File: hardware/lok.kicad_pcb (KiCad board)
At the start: 2 copper layers, 80 x 20 mm, 2 parts, among them U1 XIAO-ESP32-S3-SMD, U2 STSPIN233

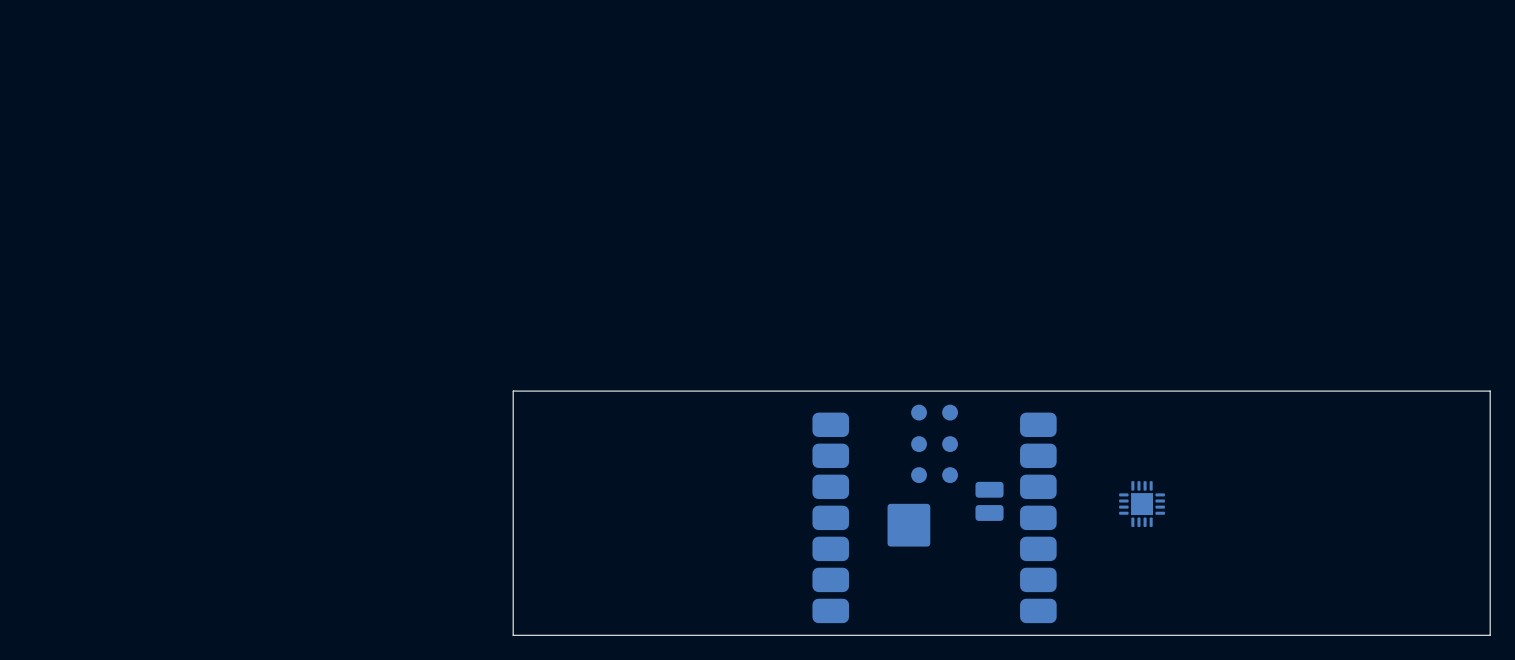
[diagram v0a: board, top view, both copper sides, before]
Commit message: update
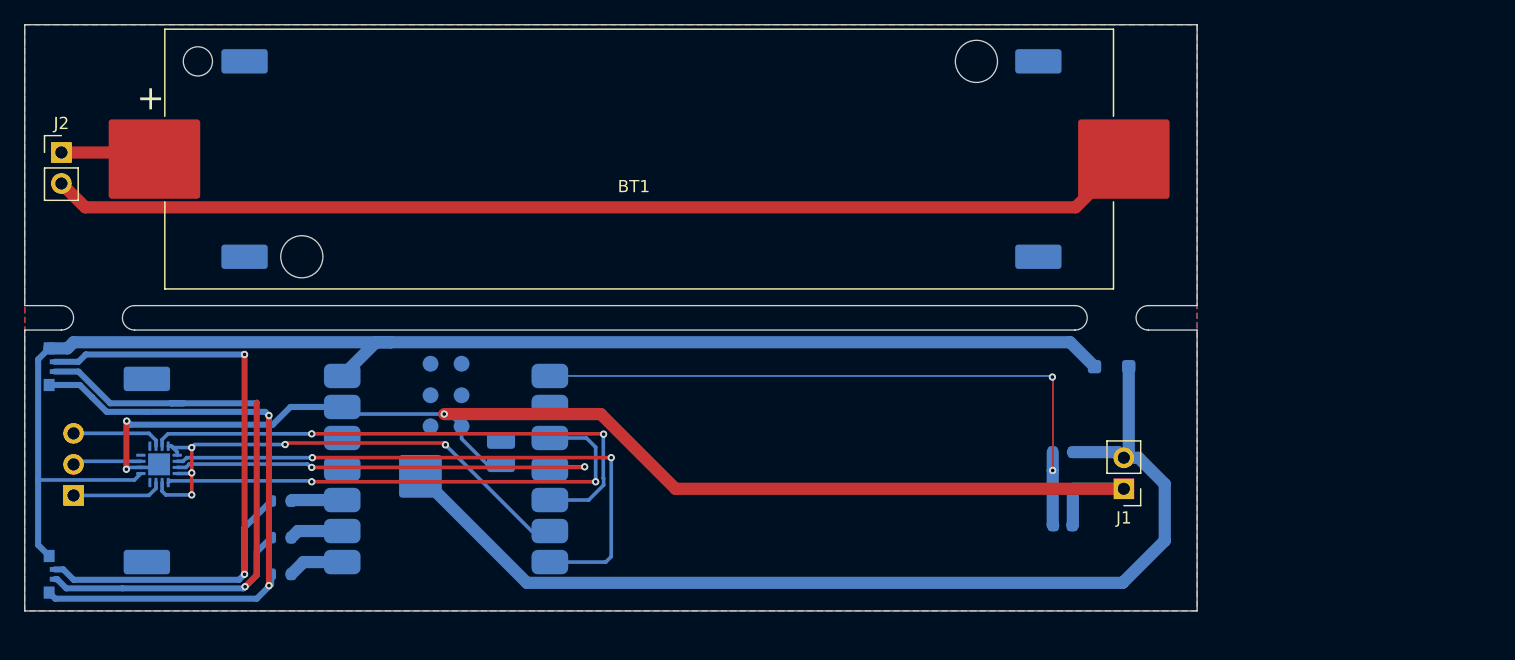
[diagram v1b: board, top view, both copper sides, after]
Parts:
- added BT1: Battery_Cell, Battery:BatteryHolder_Keystone_1042_1x18650, F.Cu at (110.3, 81.0)
- added C1: 1u, Capacitor_SMD:C_0603_1608Metric, B.Cu at (145.0, 111.0)
- added D1: D, Diode_SMD:D_SOD-123F, B.Cu at (149.0, 98.0)
- added D2: LED_ABGR, LED_SMD:LED_Kingbright_APFA3010_3x1.5mm_Horizontal, B.Cu at (62.0, 98.0)
- added D3: LED_ABGR, LED_SMD:LED_Kingbright_APFA3010_3x1.5mm_Horizontal, B.Cu at (62.0, 115.0)
- added J1: Conn_01x02_Pin, Connector_PinHeader_2.54mm:PinHeader_1x02_P2.54mm_Vertical, F.Cu at (150.0, 108.0)
- added J2: Conn_01x02_Pin, Connector_PinHeader_2.54mm:PinHeader_1x02_P2.54mm_Vertical, F.Cu at (63.0, 80.5)
- added J3: Conn_01x03_Pin, Connector_PinHeader_2.54mm:PinHeader_1x03_P2.54mm_Vertical, B.Cu at (64.0, 108.5)
- added R1: 220k, Resistor_SMD:R_0603_1608Metric, B.Cu at (145.0, 105.0)
- added R2: 47k, Resistor_SMD:R_0603_1608Metric, B.Cu at (145.0, 108.0)
- added R3: 100, Resistor_SMD:R_0603_1608Metric, B.Cu at (81.0, 109.0)
- added R4: 100, Resistor_SMD:R_0603_1608Metric, B.Cu at (81.0, 112.0)
- added R5: 100, Resistor_SMD:R_0603_1608Metric, B.Cu at (81.0, 115.0)
- added TP3: TestPoint, TestPoint:TestPoint_Keystone_5019_Miniature, B.Cu at (70.0, 114.0)
- added TP4: TestPoint, TestPoint:TestPoint_Keystone_5019_Miniature, B.Cu at (70.0, 99.0)
- added TP5: TestPoint, TestPoint:TestPoint_Keystone_5019_Miniature, B.Cu at (143.0, 73.0)
- added TP6: TestPoint, TestPoint:TestPoint_Keystone_5019_Miniature, B.Cu at (143.0, 89.0)
- added TP7: TestPoint, TestPoint:TestPoint_Keystone_5019_Miniature, B.Cu at (78.0, 89.0)
- added TP8: TestPoint, TestPoint:TestPoint_Keystone_5019_Miniature, B.Cu at (78.0, 73.0)
- moved U2 80.6 mm to (71.0, 106.0), turned to 90 degrees
- moved U1 40.2 mm to (94.5, 106.4)
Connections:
- U1 pad 1: unconnected-(U1-GPIO0_A0_D0-Pad1) -> /V_bat_meas
- U1 pad 10: unconnected-(U1-GPIO20_D9_MISO-Pad10) -> Net-(U1-GPIO20_D9_MISO)
- U1 pad 13: unconnected-(U1-GND-Pad13) -> /GND
- U1 pad 14: unconnected-(U1-5V-Pad14) -> Net-(D1-K)
- U1 pad 15: unconnected-(U1-BAT-Pad15) -> /V_bat
- U1 pad 16: unconnected-(U1-GND-Pad16) -> /GND
- U1 pad 20: unconnected-(U1-GND-Pad20) -> /GND
- U1 pad 3: unconnected-(U1-GPIO2_A2_D2-Pad3) -> Net-(U1-GPIO2_A2_D2)
- U1 pad 4: unconnected-(U1-GPIO21_D3-Pad4) -> Net-(U1-GPIO21_D3)
- U1 pad 5: unconnected-(U1-GPIO22_D4_SDA-Pad5) -> Net-(U1-GPIO22_D4_SDA)
- U1 pad 6: unconnected-(U1-GPIO23_D5_SCL-Pad6) -> Net-(U1-GPIO23_D5_SCL)
- U1 pad 7: unconnected-(U1-GPIO16_D6_TX-Pad7) -> Net-(U1-GPIO16_D6_TX)
- U1 pad 8: unconnected-(U1-GPIO17_D7_RX-Pad8) -> Net-(U1-GPIO17_D7_RX)
- U1 pad 9: unconnected-(U1-GPIO19_D8_SCK-Pad9) -> Net-(U1-GPIO19_D8_SCK)
- U2 pad 1: unconnected-(U2-INU-Pad1) -> Net-(U1-GPIO2_A2_D2)
- U2 pad 10: unconnected-(U2-OUTW-Pad10) -> Net-(J3-Pin_3)
- U2 pad 11: unconnected-(U2-INW-Pad11) -> Net-(U1-GPIO22_D4_SDA)
- U2 pad 12: unconnected-(U2-ENW-Pad12) -> Net-(U1-GPIO23_D5_SCL)
- U2 pad 13: unconnected-(U2-EN/FAULT-Pad13) -> Net-(U1-GPIO23_D5_SCL)
- U2 pad 14: unconnected-(U2-STBY/RESET-Pad14) -> Net-(U1-GPIO16_D6_TX)
- U2 pad 15: unconnected-(U2-INV-Pad15) -> Net-(U1-GPIO21_D3)
- U2 pad 16: unconnected-(U2-ENV-Pad16) -> Net-(U1-GPIO23_D5_SCL)
- U2 pad 17: Net-(U2-GND-Pad17) -> /GND
- U2 pad 2: unconnected-(U2-ENU-Pad2) -> Net-(U1-GPIO23_D5_SCL)
- U2 pad 3: unconnected-(U2-OUTU-Pad3) -> Net-(J3-Pin_1)
- U2 pad 5: unconnected-(U2-VS-Pad5) -> Net-(D1-K)
- U2 pad 6: Net-(U2-GND-Pad17) -> /GND
- U2 pad 7: unconnected-(U2-OUTV-Pad7) -> Net-(J3-Pin_2)
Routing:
- net Net-(D1-K): track 0.00 -> 118.2 mm
- net /GND: track 0.00 -> 106.1 mm, vias 0 -> 3
- net Net-(BT1--): track 0.00 -> 89.4 mm
- net /V_bat: track 0.00 -> 86.9 mm
- net Net-(D2-RK): track 0.00 -> 56.8 mm, vias 0 -> 2
- net Net-(D2-GK): track 0.00 -> 55.0 mm, vias 0 -> 1
- net /V_bat_meas: track 0.00 -> 54.9 mm, vias 0 -> 2
- net Net-(D2-BK): track 0.00 -> 52.7 mm, vias 0 -> 2
- net Net-(U1-GPIO16_D6_TX): track 0.00 -> 49.0 mm, vias 0 -> 2
- net Net-(U1-GPIO22_D4_SDA): track 0.00 -> 46.0 mm, vias 0 -> 2
- net Net-(U1-GPIO23_D5_SCL): track 0.00 -> 43.7 mm, vias 0 -> 5
- net Net-(U1-GPIO2_A2_D2): track 0.00 -> 42.0 mm, vias 0 -> 2
- net Net-(U1-GPIO21_D3): track 0.00 -> 36.5 mm, vias 0 -> 2
- net Net-(BT1-+): track 0.00 -> 7.84 mm
- net Net-(J3-Pin_3): track 0.00 -> 7.46 mm
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- added copper zone on B.Cu, net /GND
- added copper zone on F.Cu, net /GND
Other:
- board size 80 x 20 mm -> 96 x 48 mm
